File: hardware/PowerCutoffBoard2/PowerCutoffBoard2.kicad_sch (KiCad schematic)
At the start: 19 parts, among them J2 Conn_01x03, J5 XT30, J6 XT60, J7 XT60, J8 XT60, J9 XT60, K1 FBR562ND12-W, Q1 SSM3K341R, Q2 SSM3K341R

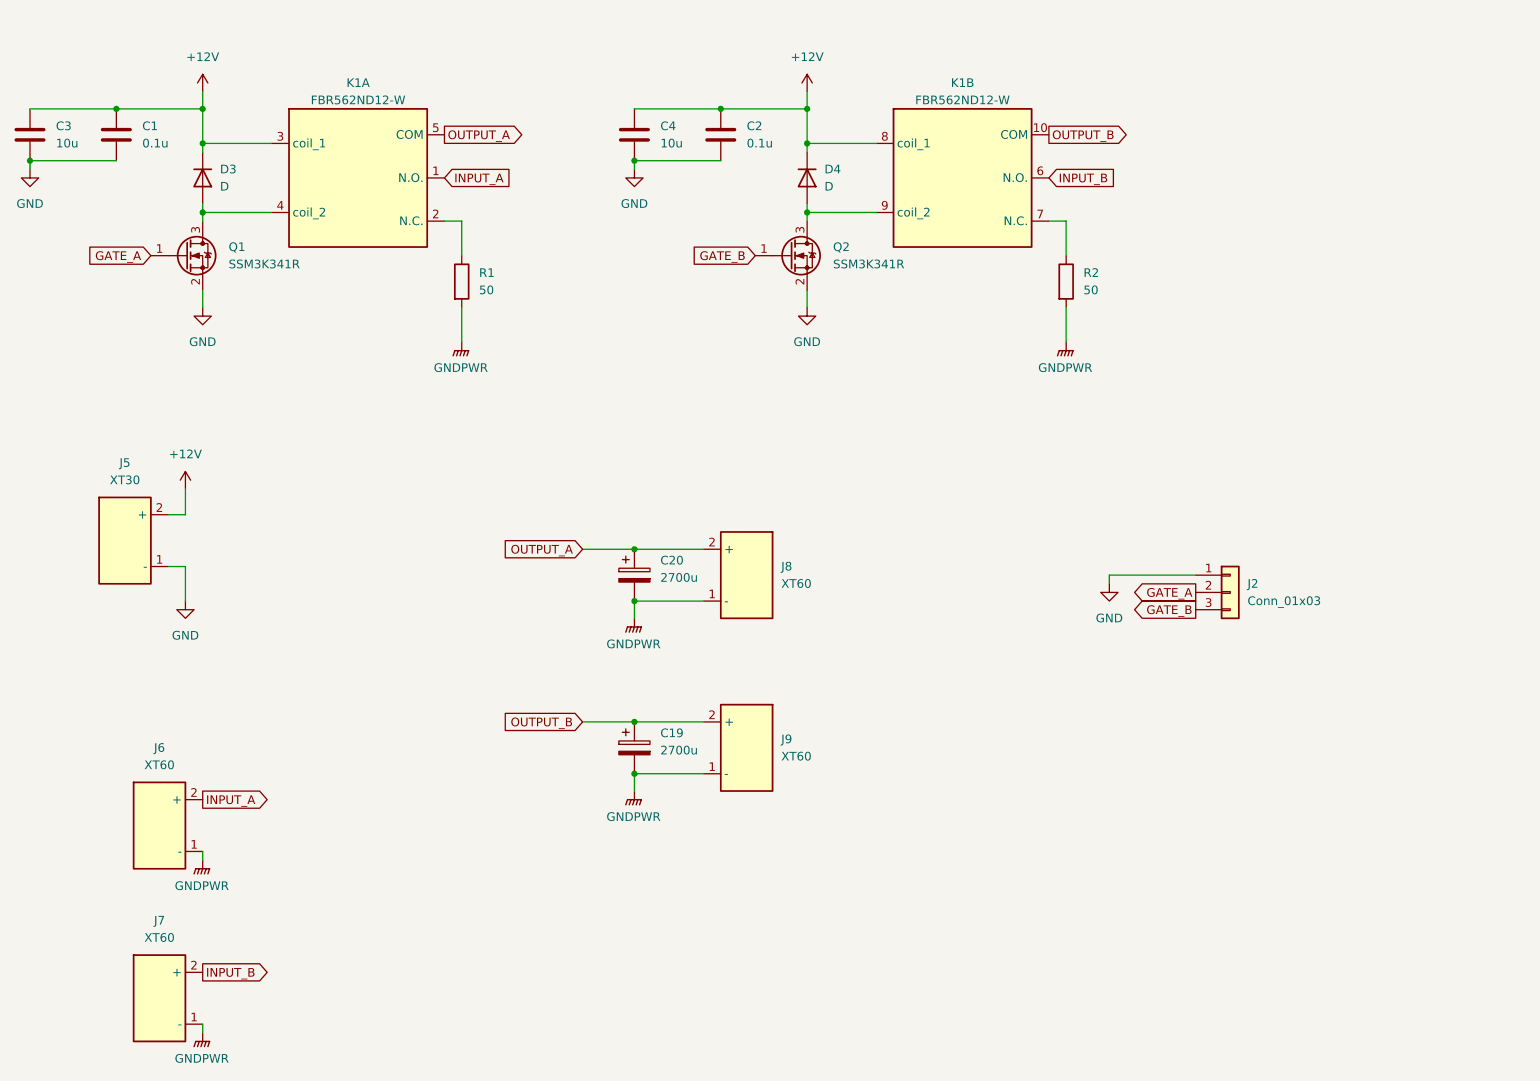
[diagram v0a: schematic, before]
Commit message: update
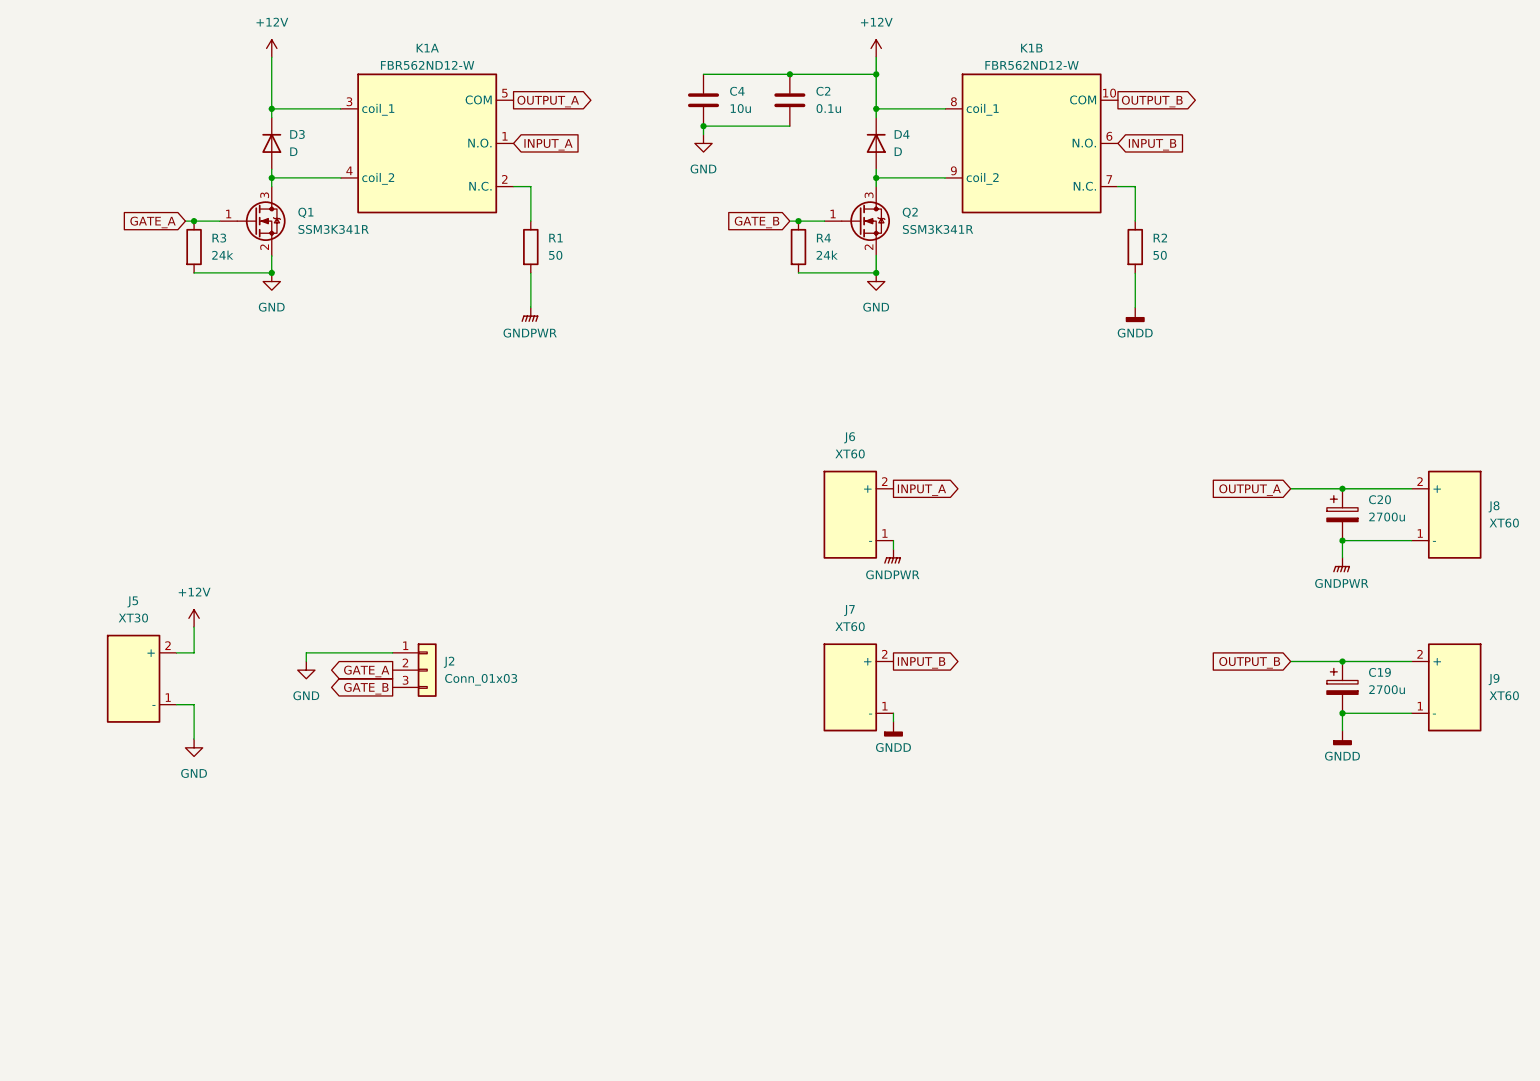
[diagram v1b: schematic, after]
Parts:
- removed C1: 0.1u, Capacitor_SMD:C_0603_1608Metric_Pad1.08x0.95mm_HandSolder, symbol Device:C
- removed C3: 10u, Capacitor_SMD:C_0805_2012Metric_Pad1.18x1.45mm_HandSolder, symbol Device:C
- added R3, R4: 24k, Resistor_SMD:R_0603_1608Metric_Pad0.98x0.95mm_HandSolder, symbol Device:R
- J5: footprint Connector_AMASS:AMASS_XT30U-M_1x02_P5.0mm_Vertical -> Connector_AMASS:AMASS_XT30PW-M_1x02_P2.50mm_Horizontal
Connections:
- net GATE_A: now also R3.1
- net GATE_B: now also R4.1
- net GND: now also R3.2, R4.2
- net GNDPWR: no longer C19.2, J7.1 (-), J9.1 (-), R2.2
- new net GNDD: C19.2, J7.1 (-), J9.1 (-), R2.2
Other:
- moved on the sheet: C19, C2, C20, C4, D3, D4, J2, J5, J6, J7, J8, J9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
